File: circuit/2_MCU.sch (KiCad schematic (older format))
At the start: 26 parts

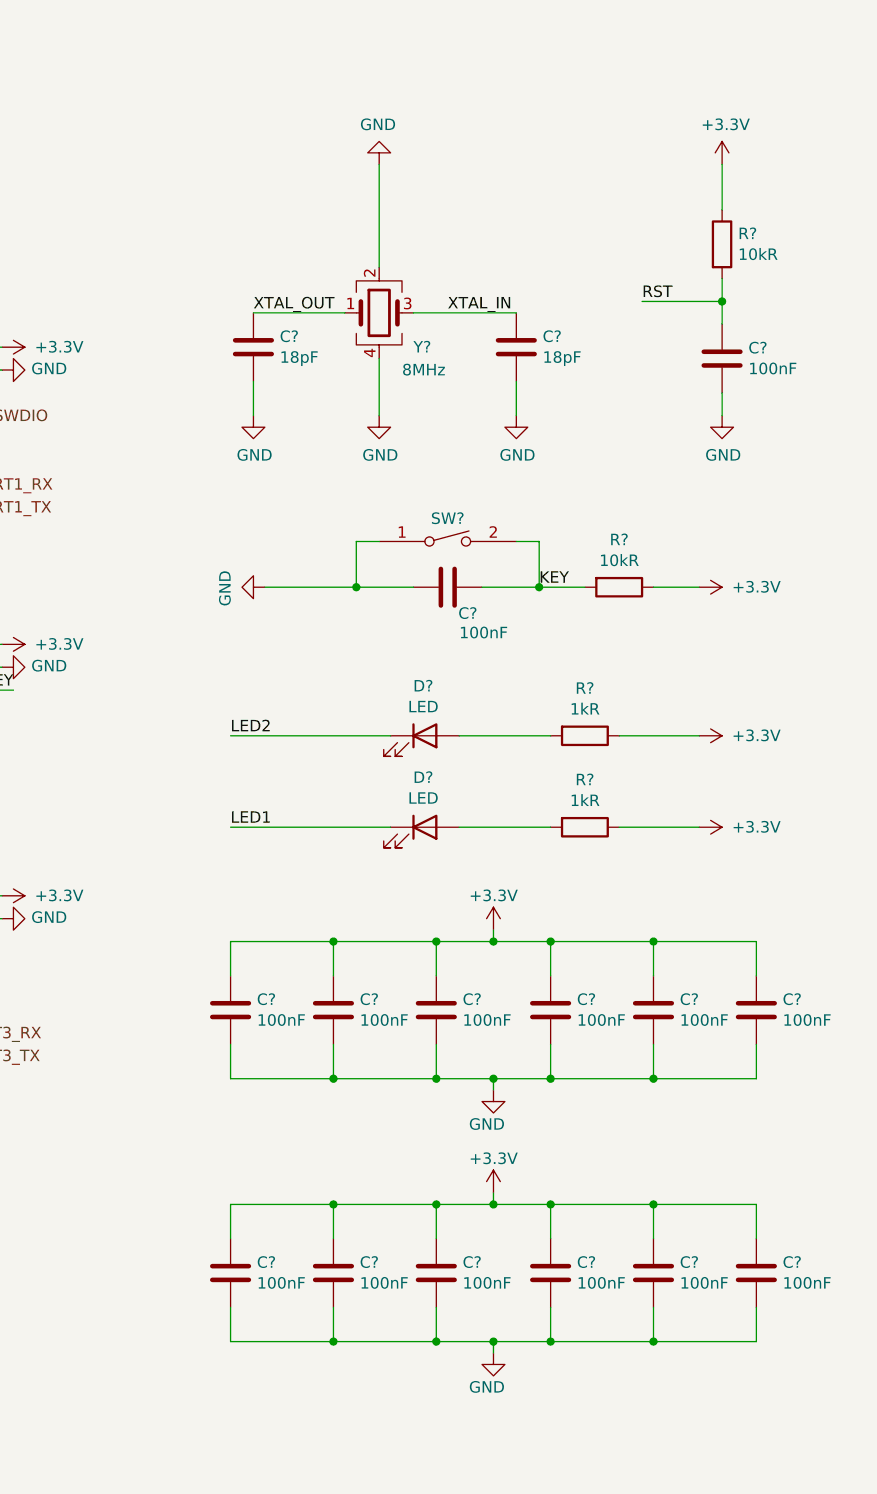
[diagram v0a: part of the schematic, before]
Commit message: Add annotations to the microcontroller subdiagram.
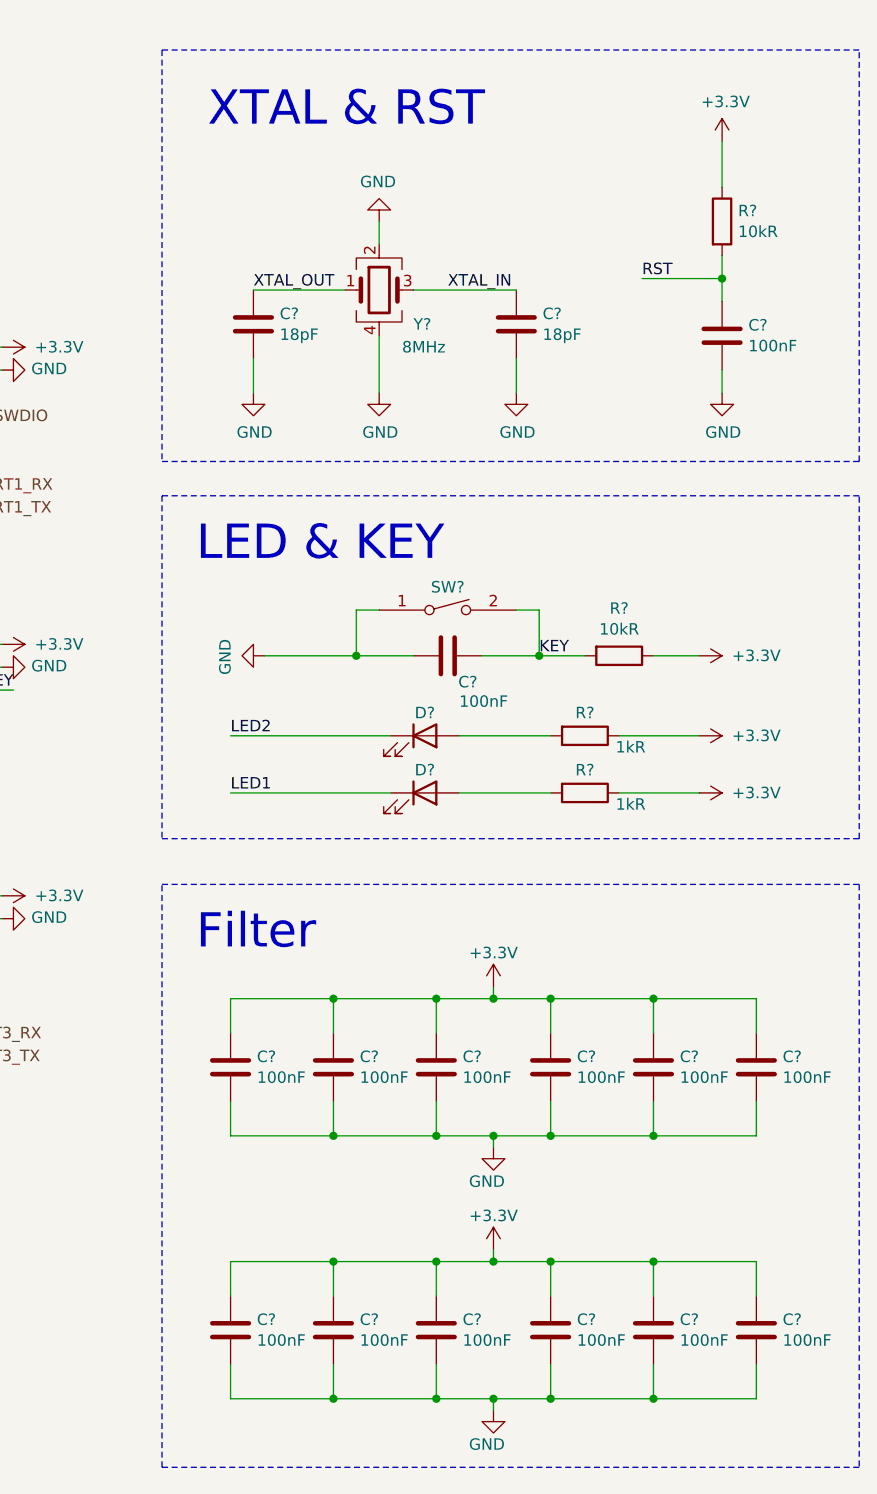
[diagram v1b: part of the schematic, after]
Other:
- note added: "Filter"
- note added: "LED & KEY"
- note added: "XTAL & RST"
- moved on the sheet: C?, D?, R?, SW?, Y?
